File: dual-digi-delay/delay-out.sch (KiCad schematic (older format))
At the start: 11 parts, among them U8 TL072

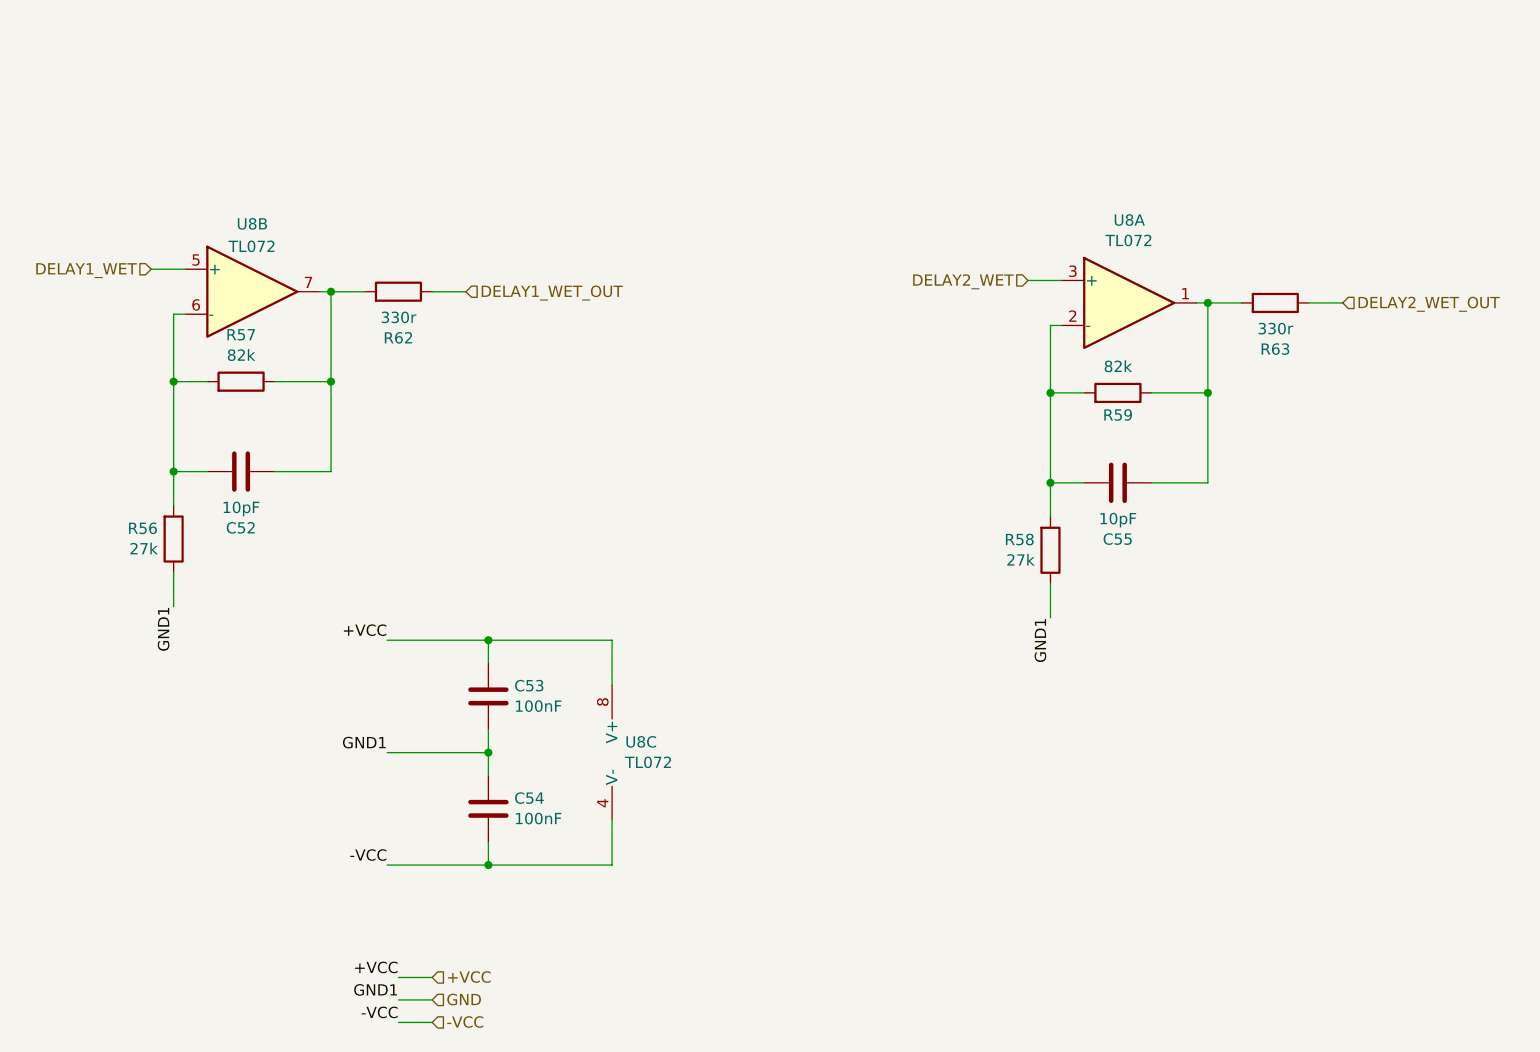
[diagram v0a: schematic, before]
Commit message: Final revision of dual digi delay
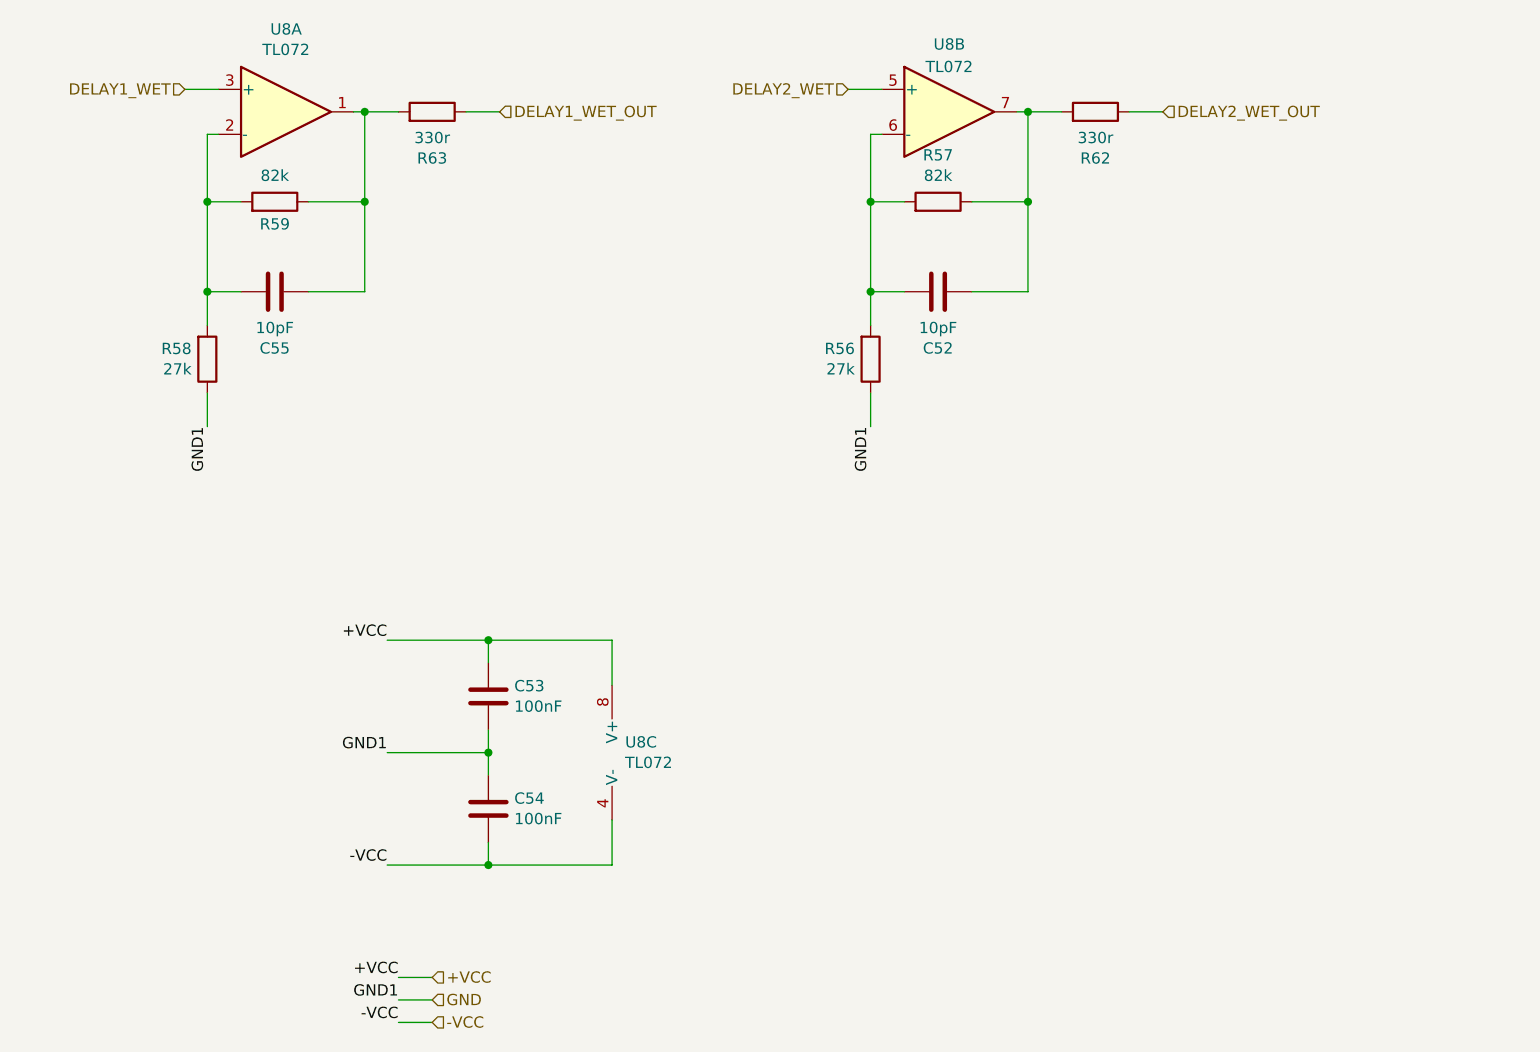
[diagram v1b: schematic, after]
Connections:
- net DELAY1_WET: now also U8.3 (+); no longer U8.5 (+)
- net DELAY1_WET_OUT: now also R63.1; no longer R62.1
- net DELAY2_WET: now also U8.5 (+); no longer U8.3 (+)
- net DELAY2_WET_OUT: now also R62.1; no longer R63.1
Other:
- moved on the sheet: C52, C55, R56, R57, R58, R59, R62, R63, U8A, U8B
